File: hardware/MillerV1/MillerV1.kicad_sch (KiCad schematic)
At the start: 290 parts, among them IC2 TUSB1106PWR, J2 Conn_02x04_Counter_Clockwise, Q1 Q12MHz/20pF/10ppm/4P/3.2x2.5mm, U1 CCGM1A1(FBGA-324), U10 RP2040(QFN-56_7x7mm_P0.4mm), U11 TPS62A02ADRLR(SOT-563-6), U12 TPS62A02ADRLR(SOT-563-6), U13 TPS62A02ADRLR(SOT-563-6), U14 TPS62A02ADRLR(SOT-563-6), U15 TPS62A02ADRLR(SOT-563-6), U16 TLV75801PDBV, U18 SiP32432DR3, U2 HX7027(SOT-23-3), U3 NA(ZD25WQ16CSIGT(SOIC-8_208mi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, U4 NA(MCP120T-300I/TT(SOT-23-3)), U5 TXB0108PWR(TSSOP-20), U6 TXB0108PWR(TSSOP-20), U7 LY68S3200SLT(SOIC-8_150mil), U8 ZD25WQ16CSIGT(SOIC-8_208mils), U9 LY68S3200SLT(SOIC-8_150mil)

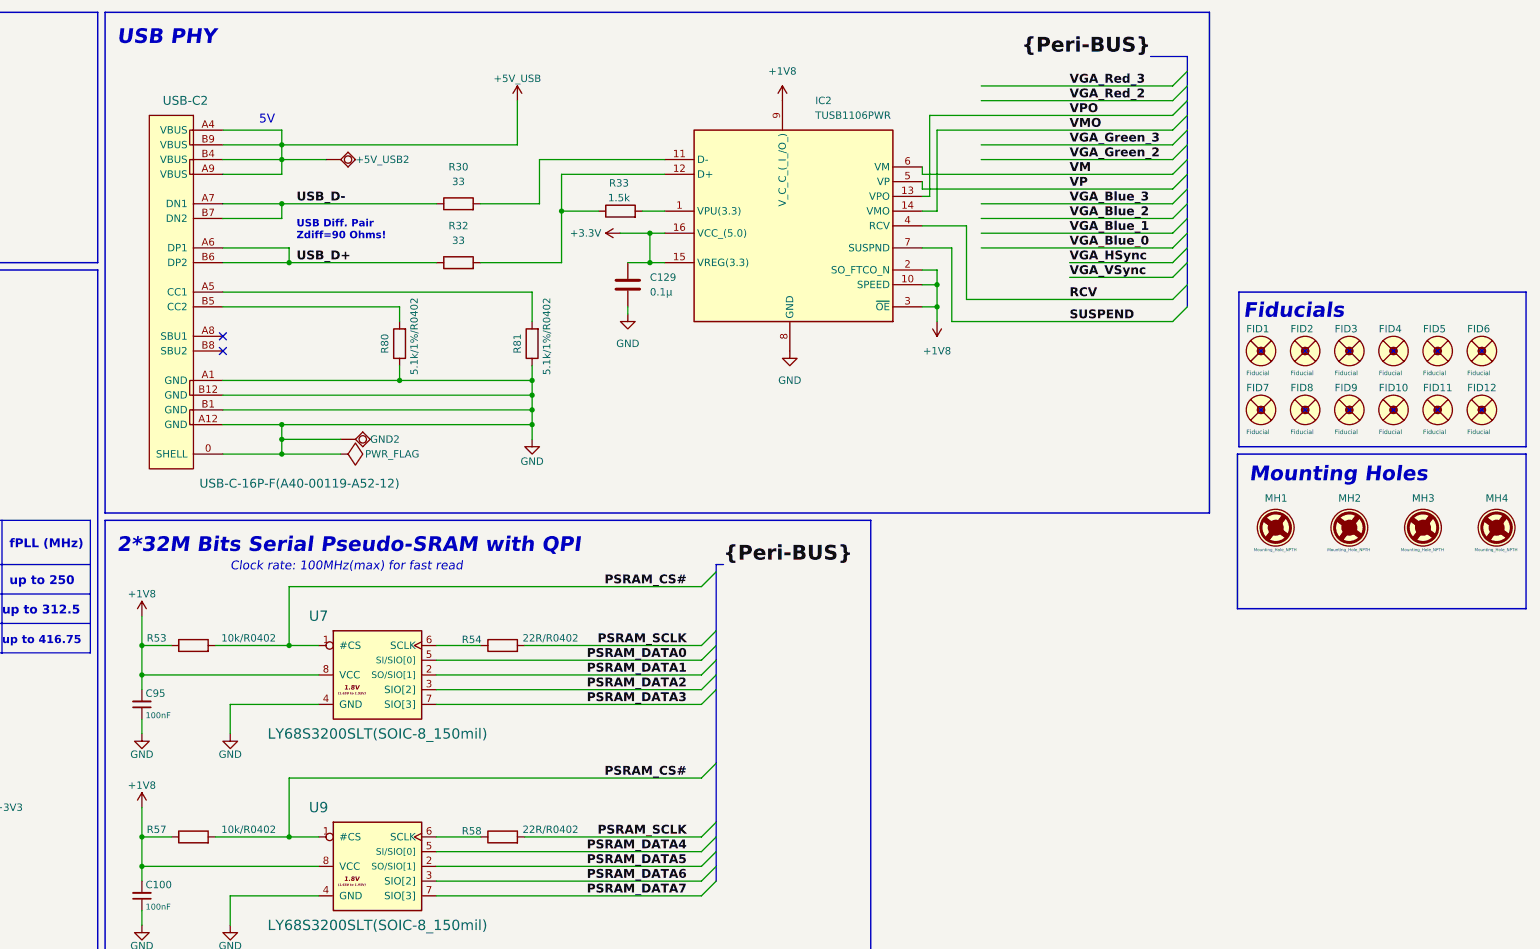
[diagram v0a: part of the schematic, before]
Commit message: Alles Kapput mach das neu in MAIN
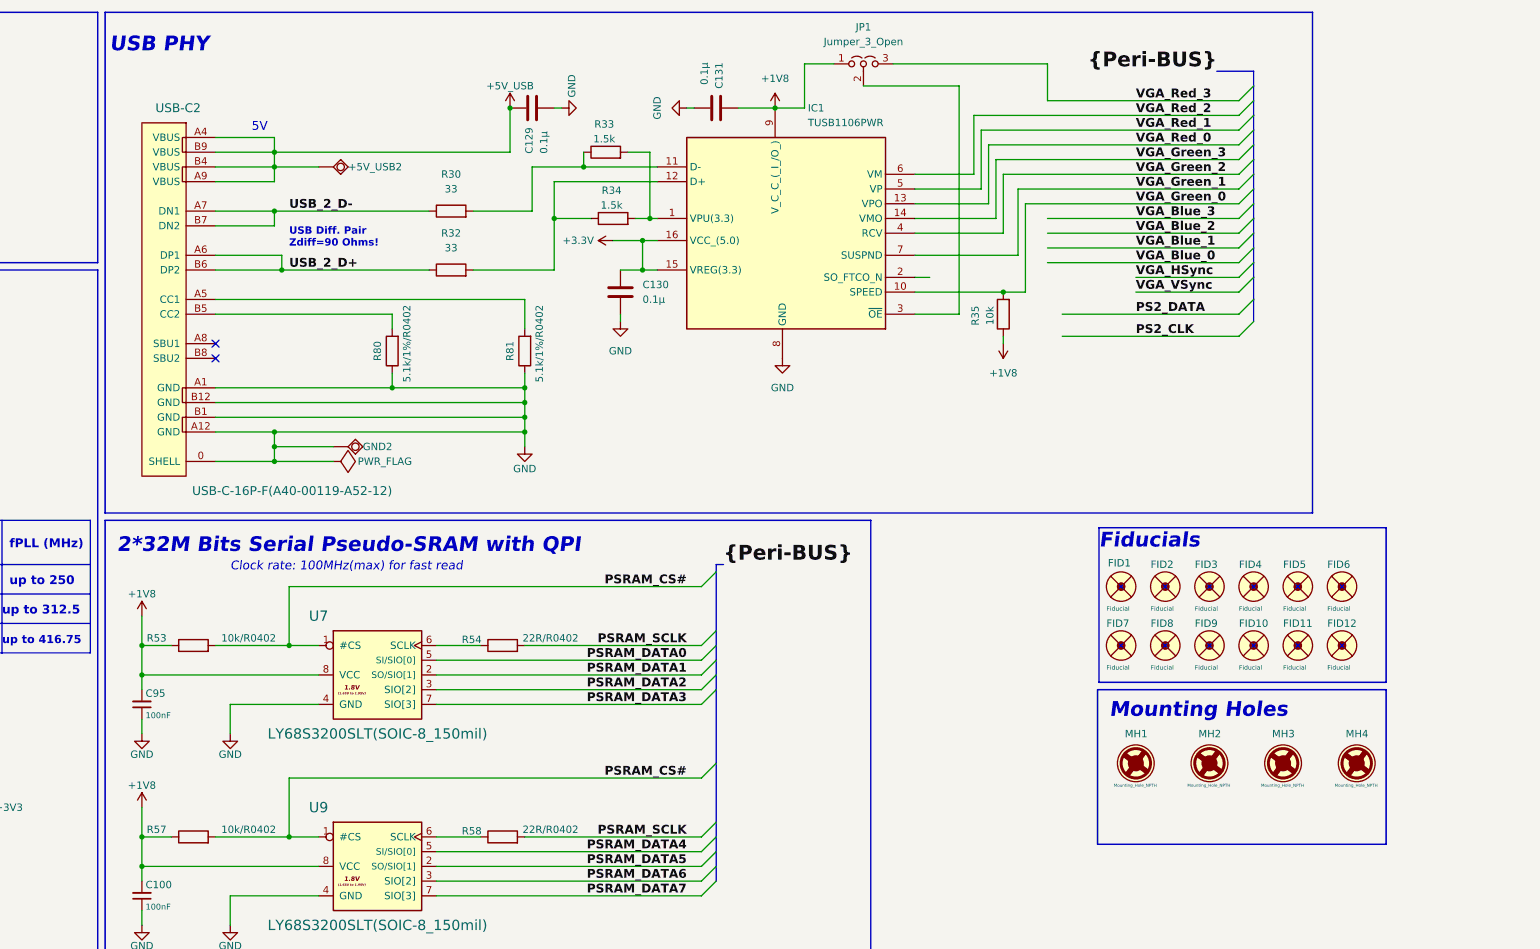
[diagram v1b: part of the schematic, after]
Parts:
- removed IC2: TUSB1106PWR, New_Libary:SOP65P640X120-16N, symbol New_Library:TUSB1106PWR
- added C130, C131: 0.1µ, New_Libary:C_0402_5MIL_DWS, symbol Device:C
- added IC1: TUSB1106PWR, New_Libary:SOP65P640X120-16N, symbol New_Library:TUSB1106PWR
- added JP1: Jumper_3_Open, Connector_PinHeader_2.54mm:PinHeader_1x03_P2.54mm_Vertical, symbol Jumper:Jumper_3_Open
- added R34: 1.5k, New_Libary:R_0402_5MIL_DWS, symbol Device:R
- added R35: 10k, New_Libary:R_0402_5MIL_DWS, symbol Device:R
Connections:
- net +1V8: now also C131.1, IC1.9 (V_C_C_(_I_/O_)), JP1.1 (A), R35.1
- net +3.3V: now also C130.1, IC1.15 (VREG(3.3)), IC1.16 (VCC_(5.0)); no longer C129.1
- net +5V_USB: now also C129.1
- net GND: now also C130.2, C131.2, IC1.8 (GND)
- net USB_D+: no longer R32.1, USB-C2.A6 (DP1), USB-C2.B6 (DP2)
- net USB_D-: no longer R30.1, USB-C2.A7 (DN1), USB-C2.B7 (DN2)
- net VGA_Green_2: now also IC1.4 (RCV)
- net VGA_Green_3: now also IC1.14 (VMO)
- net VGA_Red_2: now also IC1.6 (VM)
- net VGA_Red_3: now also JP1.3 (B)
- net at R32.2: now also IC1.12 (D+), R34.1; no longer R33.1
- net at R33.2: now also IC1.1 (VPU(3.3)), R34.2
- net at R30.2: now also R33.1, IC1.11 (D-)
- new net: IC1.3 (~{OE}), JP1.2 (C)
- new net USB_2_D+: R32.1, USB-C2.A6 (DP1), USB-C2.B6 (DP2)
- new net USB_2_D-: R30.1, USB-C2.A7 (DN1), USB-C2.B7 (DN2)
- new net VGA_Green_0: IC1.10 (SPEED), R35.2
- new net VGA_Green_1: IC1.7 (SUSPND)
- new net VGA_Red_0: IC1.13 (VPO)
- new net VGA_Red_1: IC1.5 (VP)
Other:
- moved on the sheet: FID1, FID10, FID11, FID12, FID2, FID3, FID4, FID5, FID6, FID7, FID8, FID9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
